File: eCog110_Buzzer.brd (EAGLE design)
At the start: 47.5 x 28 mm, 4 parts

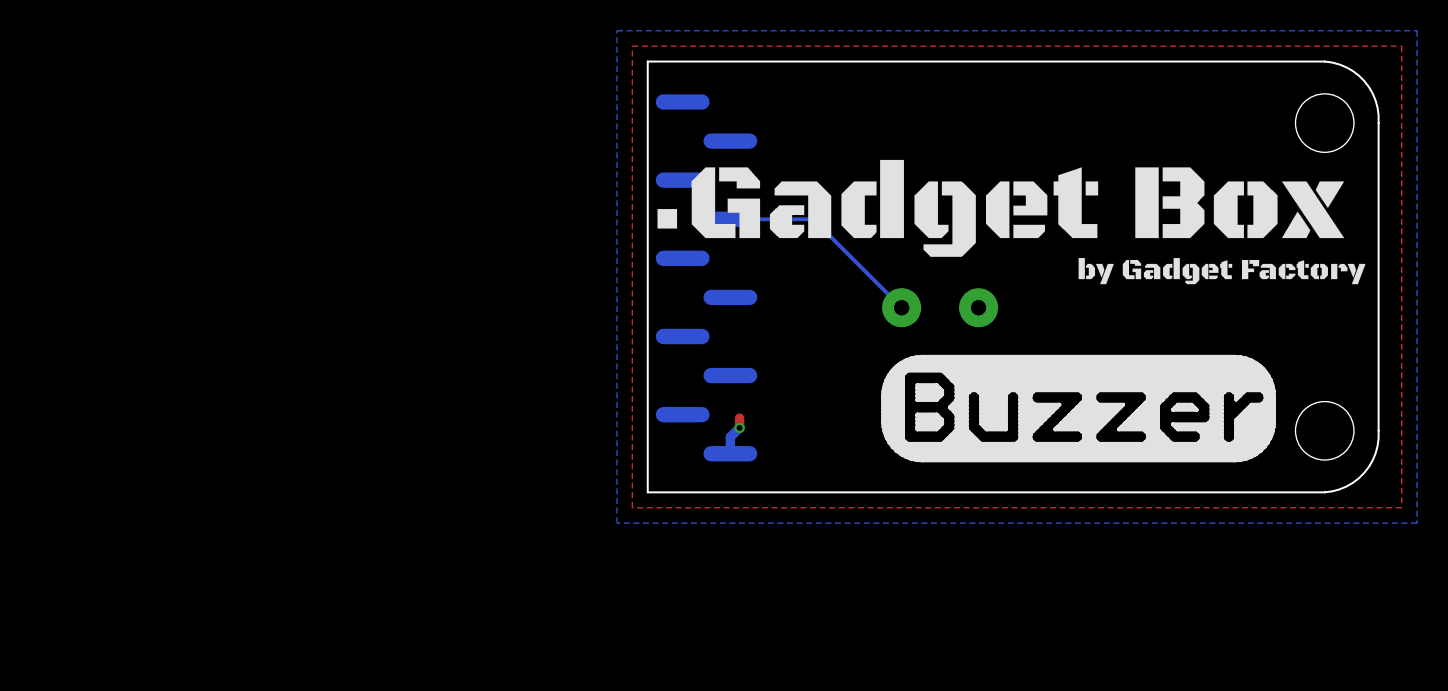
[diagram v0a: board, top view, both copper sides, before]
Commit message: All the 2.0 updates
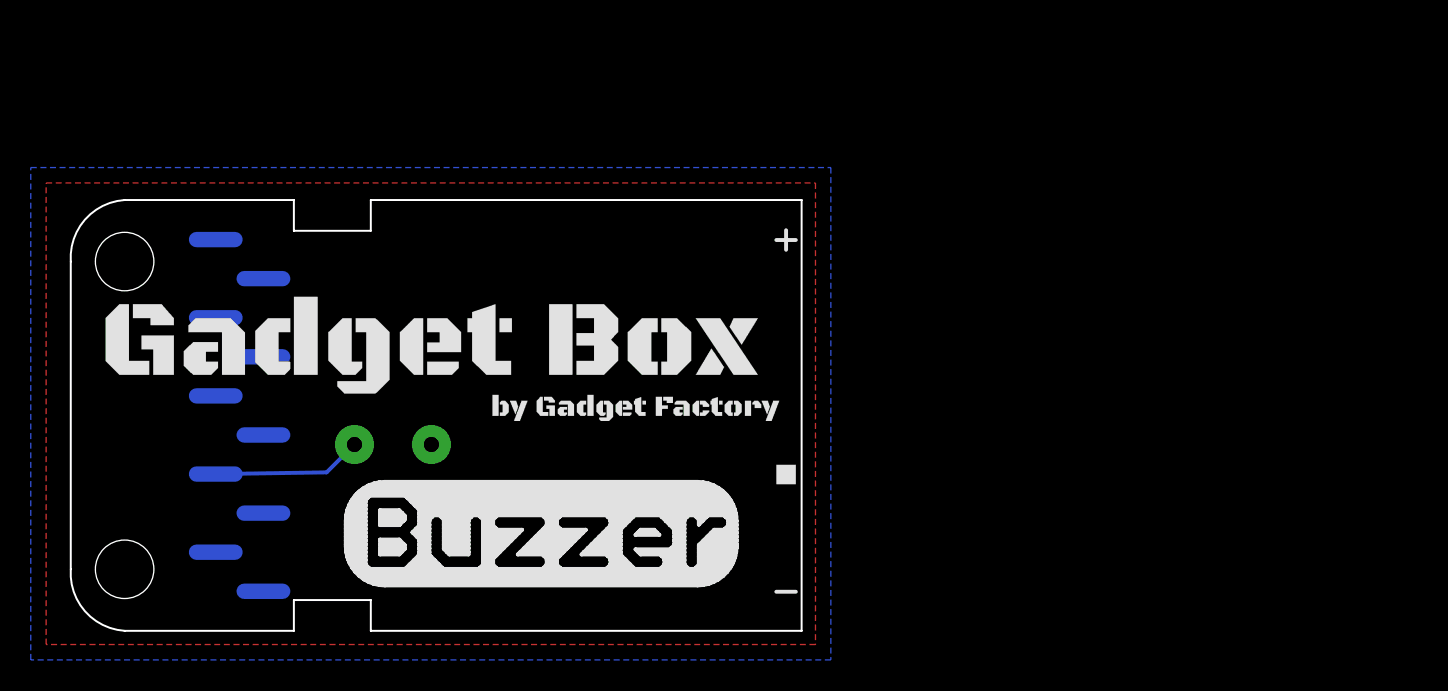
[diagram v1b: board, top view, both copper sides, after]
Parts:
- moved U$1 39.1 mm to (24.0, 18.4)
- moved ECOG 39.1 mm to (0.00, 0.00)
- moved SP1 36.7 mm to (21.4, 12.1)
- moved U$4 18.3 mm to (47.0, 10.2)
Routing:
- net N$1: track 13.5 -> 9.77 mm
- net 3V3: track 2.56 -> 0.00 mm, vias 1 -> 0
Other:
- outline, holes or cut-outs redrawn
- board text added: "2"
- board text added: "ecog110 v2.0"
- board text removed: "ecog110 v1.0"
